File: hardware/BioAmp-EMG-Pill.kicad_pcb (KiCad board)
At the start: 2 copper layers, 47.5 x 12.4 mm, 30 parts, among them J1 Conn_01x03, J3 Conn_01x04, U1 TL074

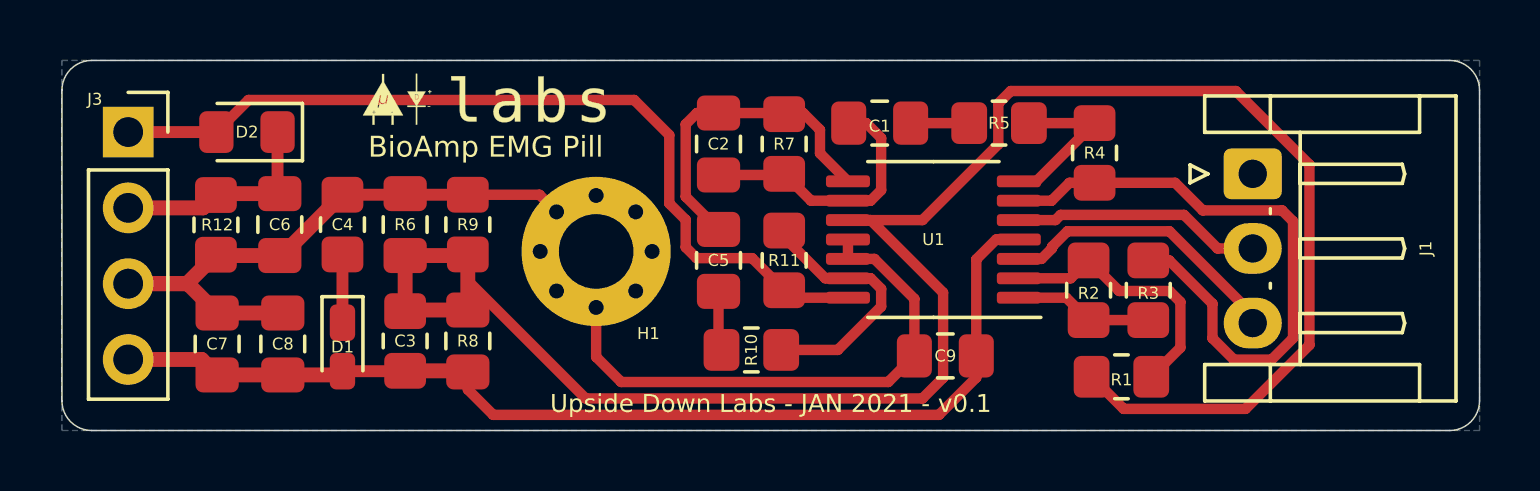
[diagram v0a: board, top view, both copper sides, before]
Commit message: Update to v0.5
Tested circuit, working great!
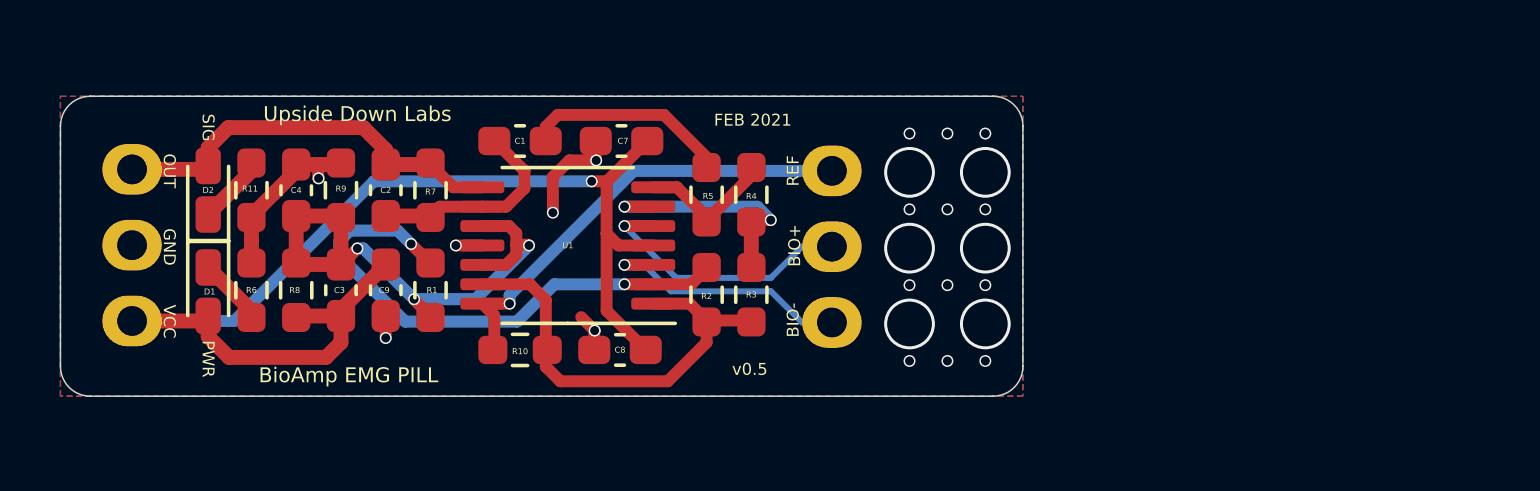
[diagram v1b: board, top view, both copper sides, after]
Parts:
- removed C5, C6: 10uf, Capacitor_SMD:C_0805_2012Metric_Pad1.18x1.45mm_HandSolder
- removed the G*** at (148.6, 96.9)
- removed the G*** at (133.1, 92.1)
- removed H1: MountingHole_Pad, MountingHole:MountingHole_2.5mm_Pad_Via
- removed J3: Conn_01x04, Connector_PinSocket_2.54mm:PinSocket_1x04_P2.54mm_Vertical
- removed R12: 10k, Resistor_SMD:R_0805_2012Metric_Pad1.20x1.40mm_HandSolder
- removed REF**: OSHW-Logo2_7.3x6mm_SilkScreen, Symbol:OSHW-Logo2_7.3x6mm_SilkScreen
- added ?: , buzzard_labels, B.Cu at (139.3, 94.5)
- added ?: , buzzard_labels, B.Cu at (138.9, 99.6)
- added ?: , buzzard_labels, B.Cu at (138.8, 97.0)
- added ?: , buzzard_labels, B.Cu at (122.5, 97.0)
- added ?: , buzzard_labels, B.Cu at (122.5, 99.6)
- added ?: , buzzard_labels, B.Cu at (122.5, 94.5)
- added G***: LOGO, udlabs:udlabs-Muscle-9.1, B.Cu at (132.9, 97.1)
- added J2: Conn_01x03, Connector_PinHeader_2.54mm:PinHeader_1x03_P2.54mm_Vertical, F.Cu at (121.2, 94.5)
- C1: value 1uf -> 2.2uf; footprint Capacitor_SMD:C_0805_2012Metric_Pad1.18x1.45mm_HandSolder -> Capacitor_SMD:C_0603_1608Metric_Pad1.08x0.95mm_HandSolder
- C2: value 1.5nf -> 100pf; footprint Capacitor_SMD:C_0805_2012Metric_Pad1.18x1.45mm_HandSolder -> Capacitor_SMD:C_0603_1608Metric_Pad1.08x0.95mm_HandSolder
- C3, C4: value 10uf -> 100n; footprint Capacitor_SMD:C_0805_2012Metric_Pad1.18x1.45mm_HandSolder -> Capacitor_SMD:C_0603_1608Metric_Pad1.08x0.95mm_HandSolder
- C7, C8, C9: footprint Capacitor_SMD:C_0805_2012Metric_Pad1.18x1.45mm_HandSolder -> Capacitor_SMD:C_0603_1608Metric_Pad1.08x0.95mm_HandSolder
- D2: value D -> LED; footprint Diode_SMD:D_0805_2012Metric_Pad1.15x1.40mm_HandSolder -> LED_SMD:LED_0603_1608Metric_Castellated
- J1: footprint Connector_JST:JST_EH_S3B-EH_1x03_P2.50mm_Horizontal -> Connector_PinHeader_2.54mm:PinHeader_1x03_P2.54mm_Vertical
- R1, R2, R3, R4, R5, R6, R8, R9: footprint Resistor_SMD:R_0805_2012Metric_Pad1.20x1.40mm_HandSolder -> Resistor_SMD:R_0603_1608Metric_Pad0.98x0.95mm_HandSolder
- R10: value 1k -> 1M; footprint Resistor_SMD:R_0805_2012Metric_Pad1.20x1.40mm_HandSolder -> Resistor_SMD:R_0603_1608Metric_Pad0.98x0.95mm_HandSolder
- R11: value 100k -> 1k; footprint Resistor_SMD:R_0805_2012Metric_Pad1.20x1.40mm_HandSolder -> Resistor_SMD:R_0603_1608Metric_Pad0.98x0.95mm_HandSolder
- R7: value 100k -> 1M; footprint Resistor_SMD:R_0805_2012Metric_Pad1.20x1.40mm_HandSolder -> Resistor_SMD:R_0603_1608Metric_Pad0.98x0.95mm_HandSolder
- moved R1 23.3 mm to (131.2, 98.5), turned to 270 degrees
- moved C9 18.9 mm to (129.8, 98.5), turned to 90 degrees
- moved R11 18.0 mm to (125.2, 95.2), turned to 90 degrees
- moved C7 15.2 mm to (137.7, 93.5), turned to 180 degrees
- moved J1 14.1 mm to (144.7, 94.5), turned to 0 degrees
- moved R3 13.3 mm to (142.0, 98.7)
- moved R2 12.8 mm to (140.5, 98.7)
- moved U1 12.3 mm to (135.8, 97.0)
- moved C1 12.1 mm to (134.2, 93.5)
- moved R7 12.0 mm to (131.2, 95.2)
- moved R4 11.6 mm to (142.0, 95.3)
- moved C8 11.3 mm to (137.6, 100.5), turned to 0 degrees
- moved C2 11.3 mm to (129.8, 95.2)
- moved R5 10.1 mm to (140.5, 95.3), turned to 270 degrees
- moved R10 7.75 mm to (134.2, 100.5)
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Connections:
- C2 pad 1: AMP2 -> OUT
- D2 pad 1: OUT -> Net-(D2-Pad1)
- D2 pad 2: RAW -> OUT
- J1 pad 1: GND -> DRL
- R10 pad 1: Net-(C5-Pad2) -> DRL
- R10 pad 2: Net-(R10-Pad2) -> DRLin
- R11 pad 1: Net-(R10-Pad2) -> GND
- R11 pad 2: RAW -> Net-(D2-Pad1)
- R2 pad 1: Net-(R2-Pad1) -> DRLin
- R3 pad 2: Net-(R2-Pad1) -> DRLin
- R7 pad 1: AMP2 -> OUT
- U1 pad 1: Net-(R2-Pad1) -> DRLin
- U1 pad 12: GND -> vRef
- U1 pad 13: Net-(R10-Pad2) -> DRLin
- U1 pad 14: RAW -> DRL
- U1 pad 8: AMP2 -> OUT
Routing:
- net vRef: track 67.5 -> 18.7 mm, vias 0 -> 3
- net GND: track 43.6 -> 12.4 mm, vias 0 -> 18
- net RAW: track 29.2 -> 0.00 mm
- net DRL: track 0.00 -> 15.4 mm, vias 0 -> 1
- net DRLin: track 0.00 -> 15.0 mm
- net Net-(R3-Pad1): track 21.1 -> 8.33 mm, vias 0 -> 2
- net AMP2: track 11.0 -> 0.00 mm
- net Net-(R1-Pad1): track 9.15 -> 18.1 mm, vias 0 -> 2
- net Net-(R10-Pad2): track 8.73 -> 0.00 mm
- net OUT: track 7.37 -> 13.8 mm
- net Net-(C1-Pad2): track 1.96 -> 7.01 mm
- net VCC: track 35.8 -> 40.7 mm, vias 0 -> 1
- net Net-(R2-Pad1): track 4.65 -> 0.00 mm
- net Net-(D2-Pad1): track 0.00 -> 2.28 mm
- net Net-(C5-Pad2): track 2.00 -> 0.00 mm
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- added copper zone on F.Cu, net GND
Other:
- board size 47.5 x 12.4 mm -> 32.2 x 10 mm
- board text added: "BIO+"
- board text added: "BIO-"
- board text added: "BioAmp EMG PILL"
- board text added: "FEB 2021"
- board text added: "PWR"
- board text added: "SIG"
- board text added: "Upside Down Labs"
- board text added: "v0.5"
- board text removed: "BioAmp EMG Pill"
- board text removed: "NEG"
- board text removed: "POS"
- board text removed: "RAW"
- board text removed: "Upside Down Labs - JAN 2021 - v0.1"

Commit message: Update to v0.6
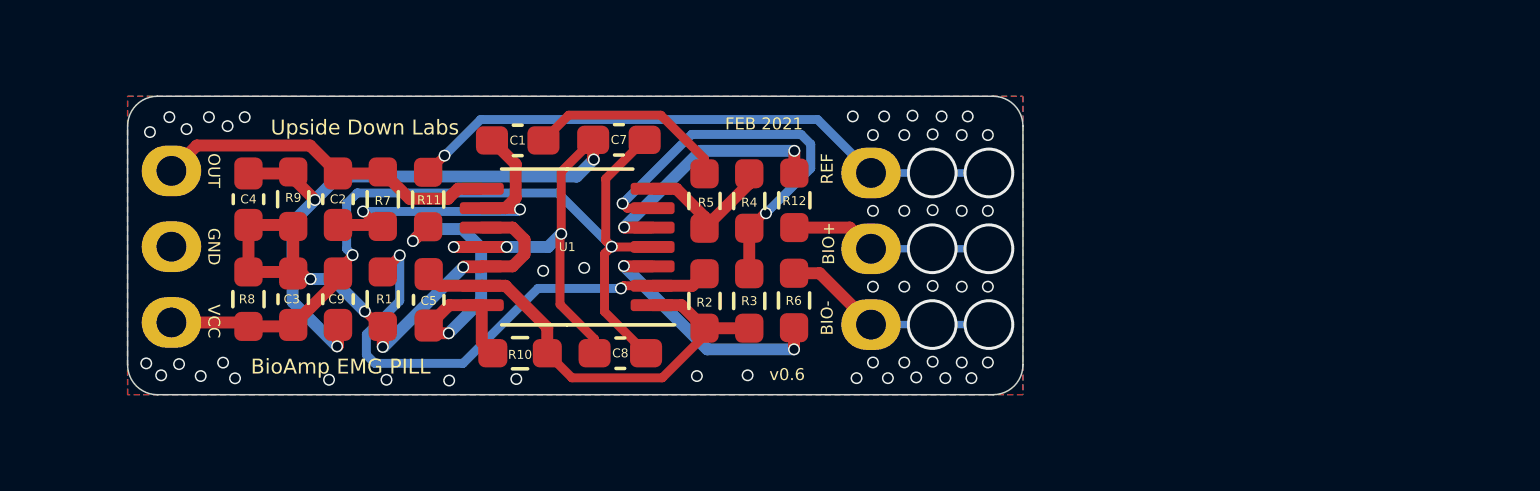
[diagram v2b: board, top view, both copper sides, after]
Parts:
- removed the ? at (139.3, 94.5)
- removed the ? at (138.9, 99.6)
- removed the ? at (138.8, 97.0)
- removed the ? at (122.5, 97.0)
- removed the ? at (122.5, 99.6)
- removed the ? at (122.5, 94.5)
- removed D1, D2: LED, LED_SMD:LED_0603_1608Metric_Castellated
- added ?: , buzzard_labels, B.Cu at (123.8, 94.5)
- added ?: , buzzard_labels, B.Cu at (123.8, 99.6)
- added ?: , buzzard_labels, B.Cu at (123.8, 97.0)
- added ?: , buzzard_labels, B.Cu at (140.2, 99.6)
- added ?: , buzzard_labels, B.Cu at (140.1, 97.0)
- added ?: , buzzard_labels, B.Cu at (140.6, 94.5)
- added C5: 100pf, Capacitor_SMD:C_0603_1608Metric_Pad1.08x0.95mm_HandSolder, F.Cu at (131.2, 98.8)
- added R12: 100k, Resistor_SMD:R_0603_1608Metric_Pad0.98x0.95mm_HandSolder, F.Cu at (143.4, 95.5)
- C8: value 10uf -> 2.2uf
- R11, R6: value 1k -> 100k
- moved R6 18.2 mm to (143.4, 98.8), turned to 90 degrees
- moved R11 5.93 mm to (131.2, 95.5), turned to 270 degrees
- moved C2 1.63 mm to (128.2, 95.5)
- moved C3 1.63 mm to (126.7, 98.8)
- moved C4 1.63 mm to (125.2, 95.5)
- moved C9 1.63 mm to (128.2, 98.8)
- moved R1 1.63 mm to (129.7, 98.8)
- moved R7 1.63 mm to (129.7, 95.5)
- moved R8 1.63 mm to (125.2, 98.8)
- moved R9 1.63 mm to (126.7, 95.5)
- moved J2 1.32 mm to (122.6, 94.5)
- moved J1 1.31 mm to (146.0, 94.6)
- moved G*** 1.23 mm to (134.1, 97.0)
- moved R4 0.22 mm to (141.9, 95.5)
- moved R5 0.22 mm to (140.4, 95.5)
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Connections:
- R10 pad 1: DRL -> Net-(C5-Pad2)
- R11 pad 1: GND -> DRL
- R11 pad 2: Net-(D2-Pad1) -> Net-(C5-Pad2)
- R6 pad 1: GND -> Net-(R6-Pad1)
- R6 pad 2: Net-(D1-Pad1) -> BIO-
- U1 pad 14: DRL -> Net-(C5-Pad2)
- U1 pad 3: BIO- -> Net-(R6-Pad1)
- U1 pad 5: BIO+ -> Net-(R12-Pad1)
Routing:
- net GND: track 12.4 -> 31.9 mm, vias 18 -> 56
- net VCC: track 40.7 -> 28.7 mm, vias 1 -> 2
- net Net-(C5-Pad2): track 0.00 -> 11.3 mm, vias 0 -> 2
- net Net-(R6-Pad1): track 0.00 -> 8.55 mm, vias 0 -> 2
- net Net-(R12-Pad1): track 0.00 -> 8.46 mm, vias 0 -> 2
- net Net-(C1-Pad1): track 7.04 -> 12.5 mm, vias 0 -> 2
- net Net-(R3-Pad1): track 8.33 -> 13.7 mm
- net DRL: track 15.4 -> 20.3 mm, vias 1 -> 3
- net Net-(D2-Pad1): track 2.28 -> 0.00 mm
- net BIO+: track 9.06 -> 6.81 mm, vias 1 -> 2
- net Net-(D1-Pad1): track 2.23 -> 0.00 mm
- net OUT: track 13.8 -> 11.7 mm
- net BIO-: track 8.71 -> 7.24 mm, vias 1 -> 2
- net Net-(R1-Pad1): track 18.1 -> 17.3 mm
- net DRLin: track 15.0 -> 15.6 mm
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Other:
- board size 32.2 x 10 mm -> 30 x 10 mm
- board text added: "v0.6"
- board text removed: "PWR"
- board text removed: "SIG"
- board text removed: "v0.5"
